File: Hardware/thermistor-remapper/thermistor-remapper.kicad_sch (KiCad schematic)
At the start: 1 part

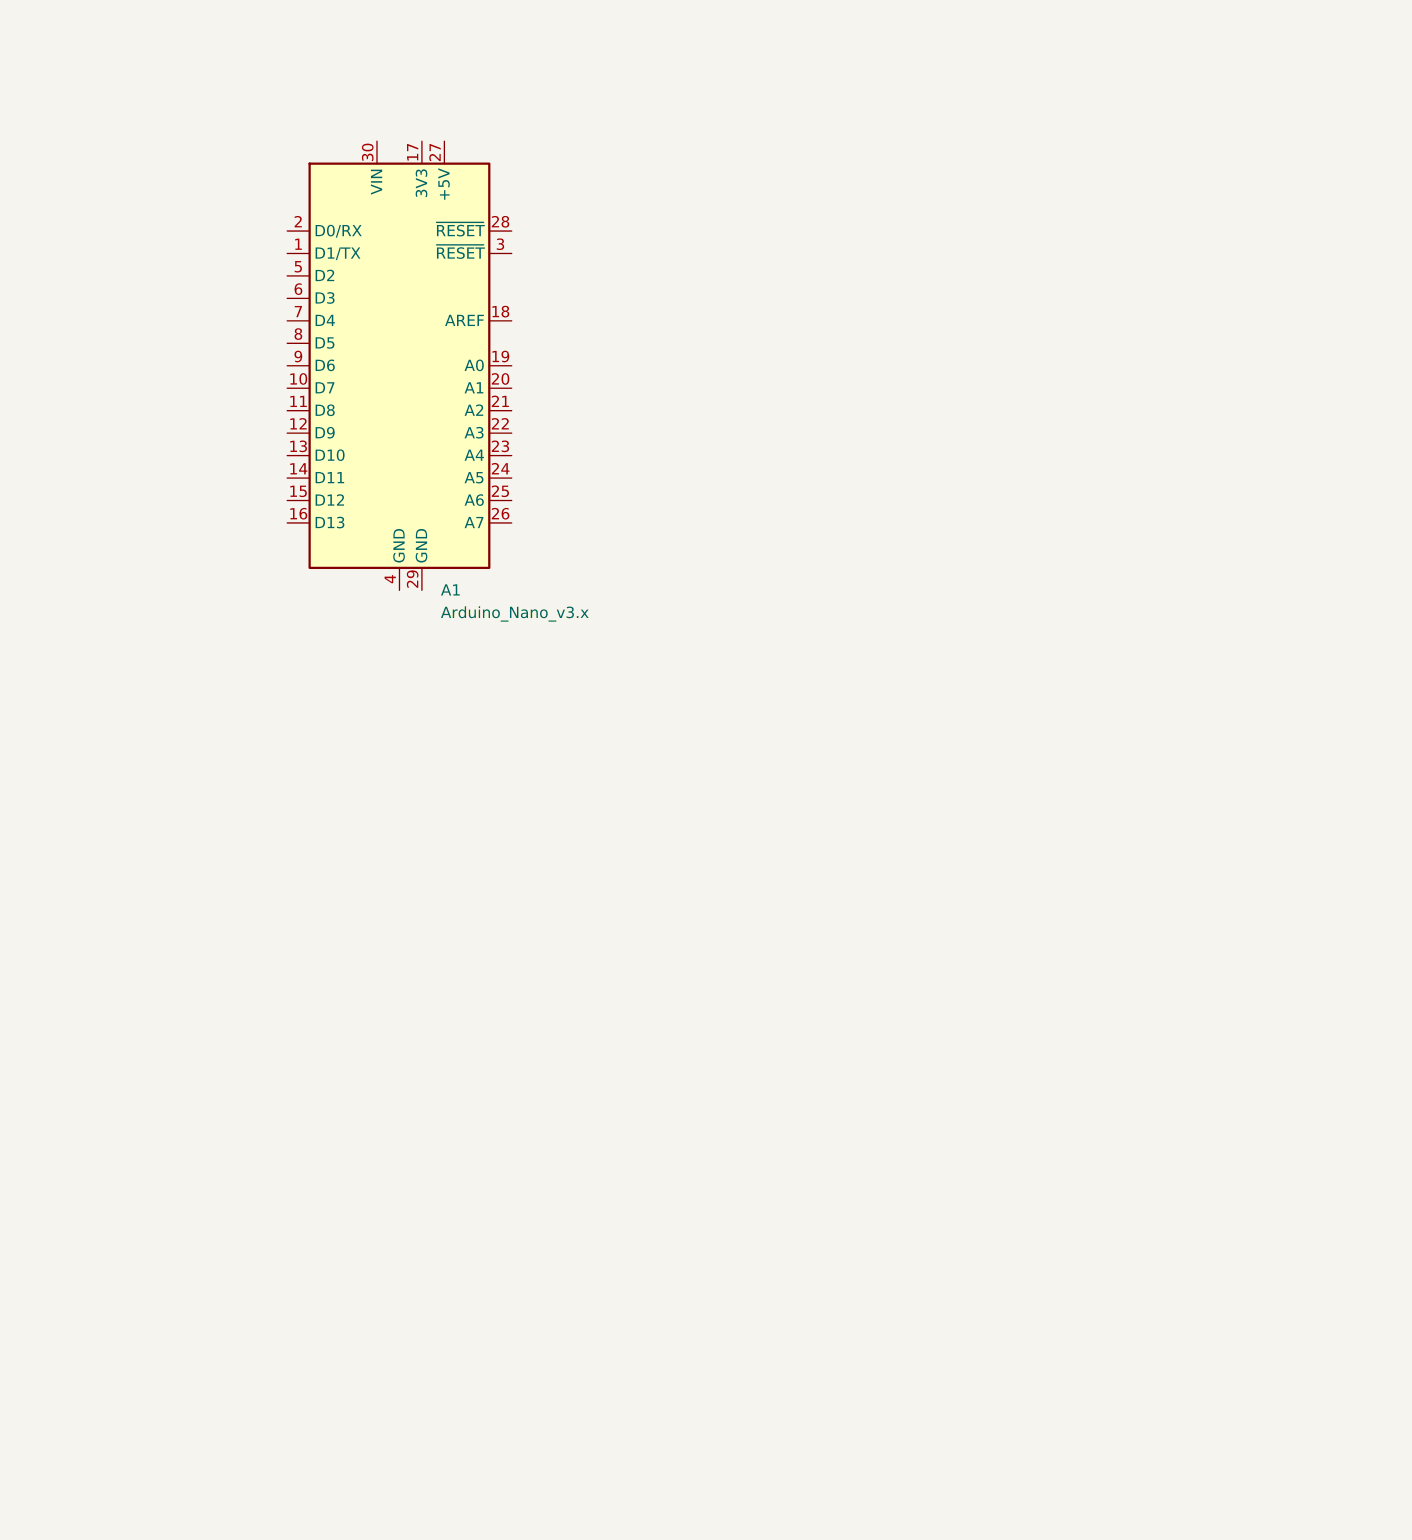
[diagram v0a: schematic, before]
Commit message: Schematic + PCB
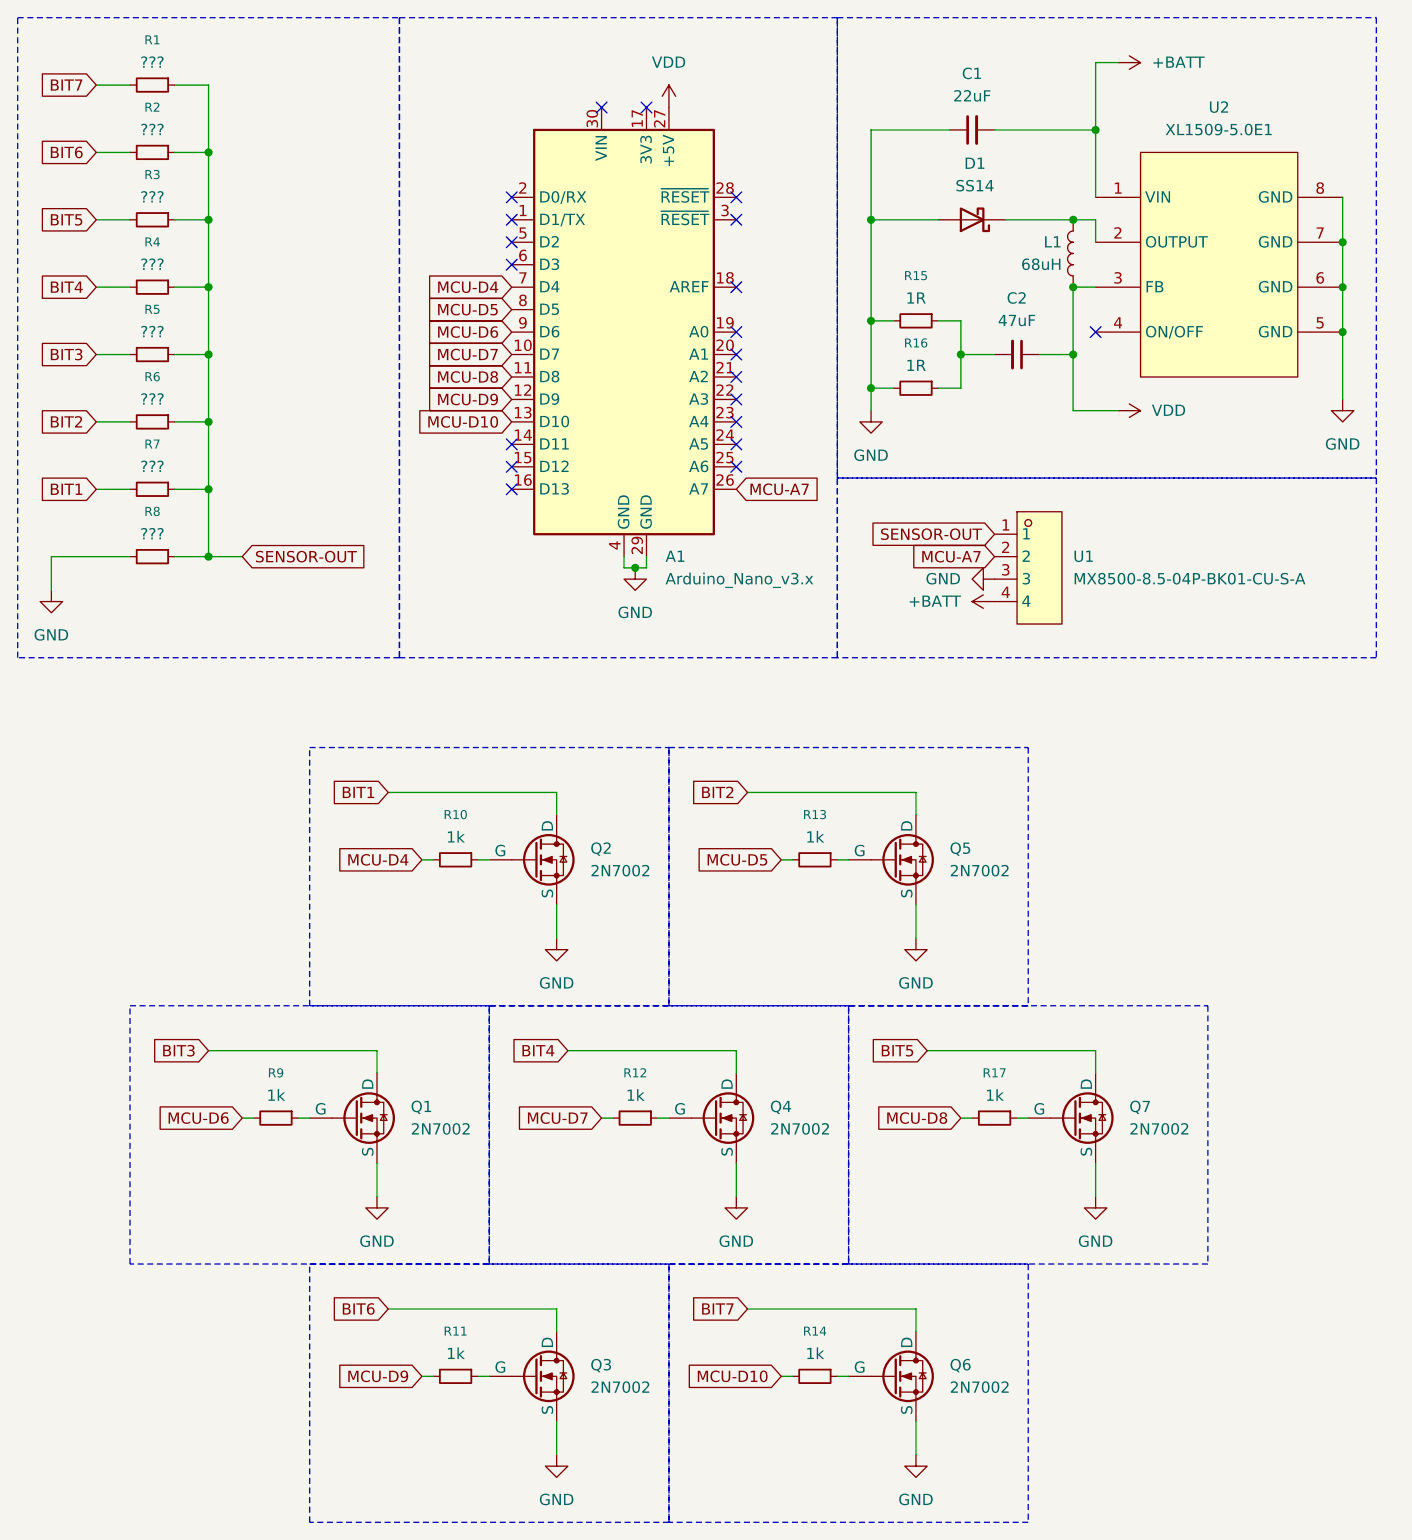
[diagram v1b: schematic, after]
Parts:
- added C1: 22uF, Capacitor_SMD:C_1206_3216Metric_Pad1.33x1.80mm_HandSolder, symbol Device:C_Small
- added C2: 47uF, Capacitor_SMD:C_1206_3216Metric_Pad1.33x1.80mm_HandSolder, symbol Device:C_Small
- added D1: SS14, Diode_SMD:D_SMA_Handsoldering, symbol Device:D_Schottky
- added L1: 68uH, Inductor_SMD:L_Bourns_SRN6045TA, symbol Device:L
- added Q1, Q2, Q3, Q4, Q5, Q6, Q7: 2N7002, Package_TO_SOT_SMD:SOT-23_Handsoldering, symbol Transistor_FET:2N7002
- added R1, R2, R3, R4, R5, R6, R7, R8: ???, Resistor_SMD:R_1206_3216Metric_Pad1.30x1.75mm_HandSolder, symbol Device:R_Small
- added R10, R11, R12, R13, R14, R17, R9: 1k, Resistor_SMD:R_1206_3216Metric_Pad1.30x1.75mm_HandSolder, symbol Device:R_Small
- added R15, R16: 1R, Resistor_SMD:R_1206_3216Metric_Pad1.30x1.75mm_HandSolder, symbol Device:R_Small
- added U1: MX8500-8.5-04P-BK01-CU-S-A, easyeda2kicad:CONN-TH_4P-P8.50_MX8500-8.5-04P-GN01-CU-S-A, symbol easyeda2kicad:MX8500-8.5-04P-BK01-CU-S-A
- added U2: XL1509-5.0E1, easyeda2kicad:SOIC-8_L5.0-W4.0-P1.27-LS6.0-BL, symbol easyeda2kicad:XL1509-5.0E1
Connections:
- net MCU-D7: now reaches A1.10 (D7)
- net MCU-D7: now also R12.2
- net MCU-D8: now reaches A1.11 (D8)
- net MCU-D8: now also R17.2
- net MCU-D9: now reaches A1.12 (D9)
- net MCU-D9: now also R11.2
- net MCU-D10: now reaches A1.13 (D10)
- net MCU-D10: now also R14.2
- net MCU-A7: now reaches A1.26 (A7)
- net MCU-A7: now also U1.2
- net VDD: now reaches A1.27 (+5V)
- net VDD: now also C2.1, L1.2, U2.3 (FB)
- net GND: now reaches A1.29 (GND)
- net GND: now also A1.4 (GND), C1.1, D1.2 (A), Q1.2 (S), Q2.2 (S), Q3.2 (S), Q4.2 (S), Q5.2 (S), Q6.2 (S), Q7.2 (S), R15.2, R16.2, R8.2, U1.3, U2.5 (GND), U2.6 (GND), U2.7 (GND), U2.8 (GND)
- net MCU-D4: now reaches A1.7 (D4)
- net MCU-D4: now also R10.2
- net MCU-D5: now reaches A1.8 (D5)
- net MCU-D5: now also R13.2
- net MCU-D6: now reaches A1.9 (D6)
- net MCU-D6: now also R9.2
- new net: Q3.1 (G), R11.1
- new net: Q2.1 (G), R10.1
- new net: Q5.1 (G), R13.1
- new net: D1.1 (K), L1.1, U2.2 (OUTPUT)
- new net: C2.2, R15.1, R16.1
- new net: Q6.1 (G), R14.1
- new net: Q7.1 (G), R17.1
- new net: Q1.1 (G), R9.1
- new net: Q4.1 (G), R12.1
- new net +BATT: C1.2, U1.4, U2.1 (VIN)
- new net BIT1: Q2.3 (D), R7.2
- new net BIT2: Q5.3 (D), R6.2
- new net BIT3: Q1.3 (D), R5.2
- new net BIT4: Q4.3 (D), R4.2
- new net BIT5: Q7.3 (D), R3.2
- new net BIT6: Q3.3 (D), R2.2
- new net BIT7: Q6.3 (D), R1.2
- new net SENSOR-OUT: R1.1, R2.1, R3.1, R4.1, R5.1, R6.1, R7.1, R8.1, U1.1
- no-connect marks 0 -> 20
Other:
- moved on the sheet: A1

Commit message: Change resistors to 0806
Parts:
- R1, R10, R11, R12, R13, R14, R15, R16, R17, R2, R3, R4, R5, R6, R7, R8, R9: footprint Resistor_SMD:R_1206_3216Metric_Pad1.30x1.75mm_HandSolder -> Resistor_SMD:R_0805_2012Metric_Pad1.20x1.40mm_HandSolder
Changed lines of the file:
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@@
 			)
 		)
-		(property "Footprint" "Resistor_SMD:R_1206_3216Metric_Pad1.30x1.75mm_HandSolder"
+		(property "Footprint" "Resistor_SMD:R_0805_2012Metric_Pad1.20x1.40mm_HandSolder"
 			(at 115.57 55.88 0)
 			(effects
@@
 			)
 		)
-		(property "Footprint" "Resistor_SMD:R_1206_3216Metric_Pad1.30x1.75mm_HandSolder"
+		(property "Footprint" "Resistor_SMD:R_0805_2012Metric_Pad1.20x1.40mm_HandSolder"
 			(at 104.14 167.64 0)
 			(effects
@@
 			)
 		)
-		(property "Footprint" "Resistor_SMD:R_1206_3216Metric_Pad1.30x1.75mm_HandSolder"
+		(property "Footprint" "Resistor_SMD:R_0805_2012Metric_Pad1.20x1.40mm_HandSolder"
 			(at 29.21 74.93 0)
 			(effects
@@
 			)
 		)
-		(property "Footprint" "Resistor_SMD:R_1206_3216Metric_Pad1.30x1.75mm_HandSolder"
+		(property "Footprint" "Resistor_SMD:R_0805_2012Metric_Pad1.20x1.40mm_HandSolder"
 			(at 29.21 29.21 0)
 			(effects
@@
 			)
 		)
-		(property "Footprint" "Resistor_SMD:R_1206_3216Metric_Pad1.30x1.75mm_HandSolder"
+		(property "Footprint" "Resistor_SMD:R_0805_2012Metric_Pad1.20x1.40mm_HandSolder"
 			(at 29.21 44.45 0)
 			(effects
@@
 			)
 		)
-		(property "Footprint" "Resistor_SMD:R_1206_3216Metric_Pad1.30x1.75mm_HandSolder"
+		(property "Footprint" "Resistor_SMD:R_0805_2012Metric_Pad1.20x1.40mm_HandSolder"
 			(at 29.21 21.59 0)
 			(effects
@@
 			)
 		)
-		(property "Footprint" "Resistor_SMD:R_1206_3216Metric_Pad1.30x1.75mm_HandSolder"
+		(property "Footprint" "Resistor_SMD:R_0805_2012Metric_Pad1.20x1.40mm_HandSolder"
 			(at 29.21 59.69 0)
 			(effects
@@
 			)
 		)
-		(property "Footprint" "Resistor_SMD:R_1206_3216Metric_Pad1.30x1.75mm_HandSolder"
+		(property "Footprint" "Resistor_SMD:R_0805_2012Metric_Pad1.20x1.40mm_HandSolder"
 			(at 124.46 138.43 0)
 			(effects
@@
 			)
 		)
-		(property "Footprint" "Resistor_SMD:R_1206_3216Metric_Pad1.30x1.75mm_HandSolder"
+		(property "Footprint" "Resistor_SMD:R_0805_2012Metric_Pad1.20x1.40mm_HandSolder"
 			(at 43.18 138.43 0)
 			(effects
@@
 			)
 		)
-		(property "Footprint" "Resistor_SMD:R_1206_3216Metric_Pad1.30x1.75mm_HandSolder"
+		(property "Footprint" "Resistor_SMD:R_0805_2012Metric_Pad1.20x1.40mm_HandSolder"
 			(at 115.57 48.26 0)
 			(effects
@@
 			)
 		)
-		(property "Footprint" "Resistor_SMD:R_1206_3216Metric_Pad1.30x1.75mm_HandSolder"
+		(property "Footprint" "Resistor_SMD:R_0805_2012Metric_Pad1.20x1.40mm_HandSolder"
 			(at 83.82 138.43 0)
 			(effects
@@
 			)
 		)
-		(property "Footprint" "Resistor_SMD:R_1206_3216Metric_Pad1.30x1.75mm_HandSolder"
+		(property "Footprint" "Resistor_SMD:R_0805_2012Metric_Pad1.20x1.40mm_HandSolder"
 			(at 63.5 167.64 0)
 			(effects
@@
 			)
 		)
-		(property "Footprint" "Resistor_SMD:R_1206_3216Metric_Pad1.30x1.75mm_HandSolder"
+		(property "Footprint" "Resistor_SMD:R_0805_2012Metric_Pad1.20x1.40mm_HandSolder"
 			(at 29.21 36.83 0)
 			(effects
@@
 			)
 		)
-		(property "Footprint" "Resistor_SMD:R_1206_3216Metric_Pad1.30x1.75mm_HandSolder"
+		(property "Footprint" "Resistor_SMD:R_0805_2012Metric_Pad1.20x1.40mm_HandSolder"
 			(at 29.21 52.07 0)
 			(effects
@@
 			)
 		)
-		(property "Footprint" "Resistor_SMD:R_1206_3216Metric_Pad1.30x1.75mm_HandSolder"
+		(property "Footprint" "Resistor_SMD:R_0805_2012Metric_Pad1.20x1.40mm_HandSolder"
 			(at 29.21 67.31 0)
 			(effects
@@
 			)
 		)
-		(property "Footprint" "Resistor_SMD:R_1206_3216Metric_Pad1.30x1.75mm_HandSolder"
+		(property "Footprint" "Resistor_SMD:R_0805_2012Metric_Pad1.20x1.40mm_HandSolder"
 			(at 63.5 109.22 0)
 			(effects
@@
 			)
 		)
-		(property "Footprint" "Resistor_SMD:R_1206_3216Metric_Pad1.30x1.75mm_HandSolder"
+		(property "Footprint" "Resistor_SMD:R_0805_2012Metric_Pad1.20x1.40mm_HandSolder"
 			(at 104.14 109.22 0)
 			(effects
